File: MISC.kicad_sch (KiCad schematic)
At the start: 0 parts

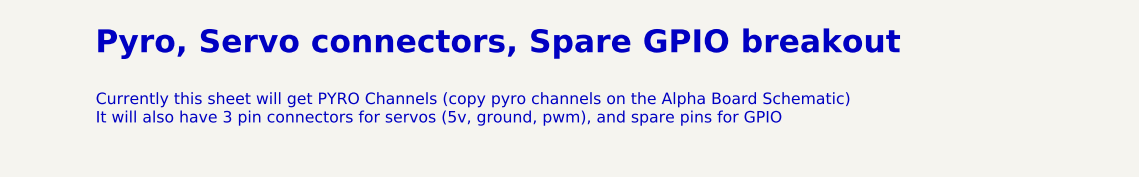
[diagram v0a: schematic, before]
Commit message: changes
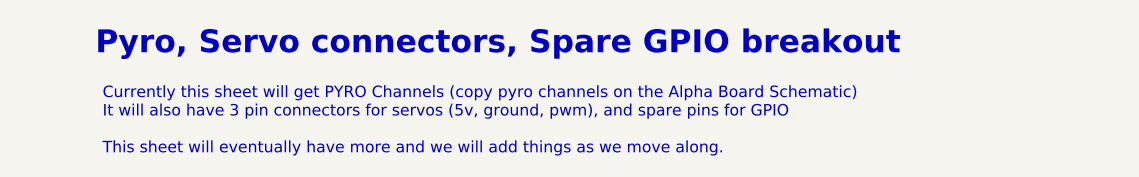
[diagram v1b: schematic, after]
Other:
- note added: "Currently this sheet will get PYRO Channels (copy pyro channels on the Alpha Board Schematic) It will also have 3 pin connectors for servos (5v, ground, pwm), and spare pins for GPIO This sheet will eventually have more and we will add things as we move along."
- note removed: "Currently this sheet will get PYRO Channels (copy pyro channels on the Alpha Board Schematic) It will also have 3 pin connectors for servos (5v, ground, pwm), and spare pins for GPIO"
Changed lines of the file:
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@@
 		)
 	)
-	(text "Currently this sheet will get PYRO Channels (copy pyro channels on the Alpha Board Schematic)\nIt will also have 3 pin connectors for servos (5v, ground, pwm), and spare pins for GPIO"
+	(text "Currently this sheet will get PYRO Channels (copy pyro channels on the Alpha Board Schematic)\nIt will also have 3 pin connectors for servos (5v, ground, pwm), and spare pins for GPIO\n\nThis sheet will eventually have more and we will add things as we move along."
 		(exclude_from_sim no)
-		(at 14.732 24.892 0)
+		(at 15.494 26.162 0)
 		(effects
 			(font
